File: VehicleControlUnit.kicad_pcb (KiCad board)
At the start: 4 copper layers, 95 x 100 mm, 99 parts, among them Con1 LED, Con2 LED, J1 Conn_01x02, J10 CAR_CAN_OUT, J11 CAR_CAN_Breakout, J12 USB_C_Receptacle_USB2.0_16P, J13 UART_Breakout, J14 Conn_01x04, J15 Conn_01x04, J16 IO_Breakout, J2 Precharge_Ready, J4 Precharge+_Conn, J5 Precharge-_Conn, J6 MOTOR_CAN_IN, J7 MOTOR_CAN_OUT, J8 MOTOR_CAN_Breakout, J9 CAR_CAN_IN, Q1 Q_PMOS_GDS, Q2 IRLML0030, Q3 IRLML0030, SW1 RESET, SW2 BOOT, U1 TLV1117LV33DCYR, U3 ESP32-C6-MINI-1/U, U4 TCMT1106, U5 TCMT1106

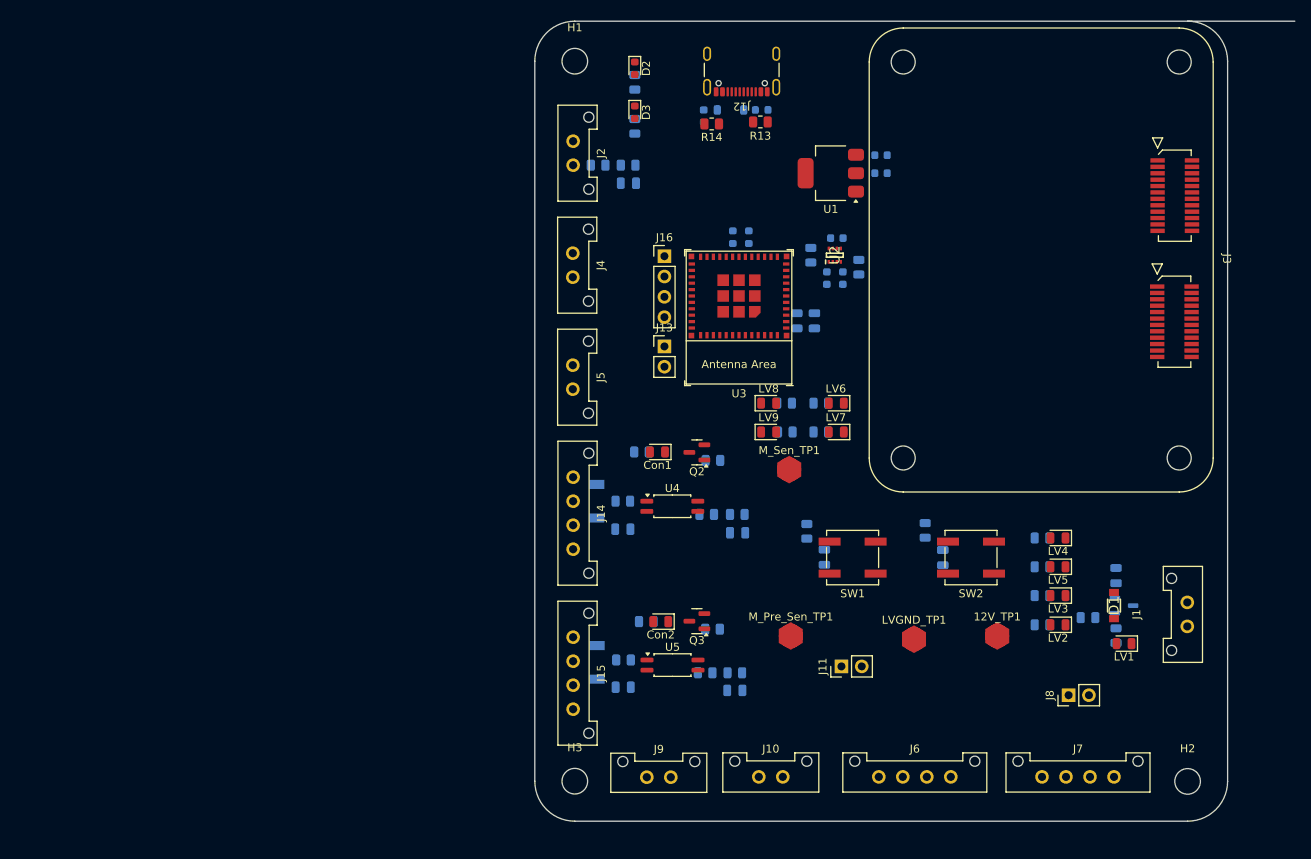
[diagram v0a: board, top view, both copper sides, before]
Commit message: first revision
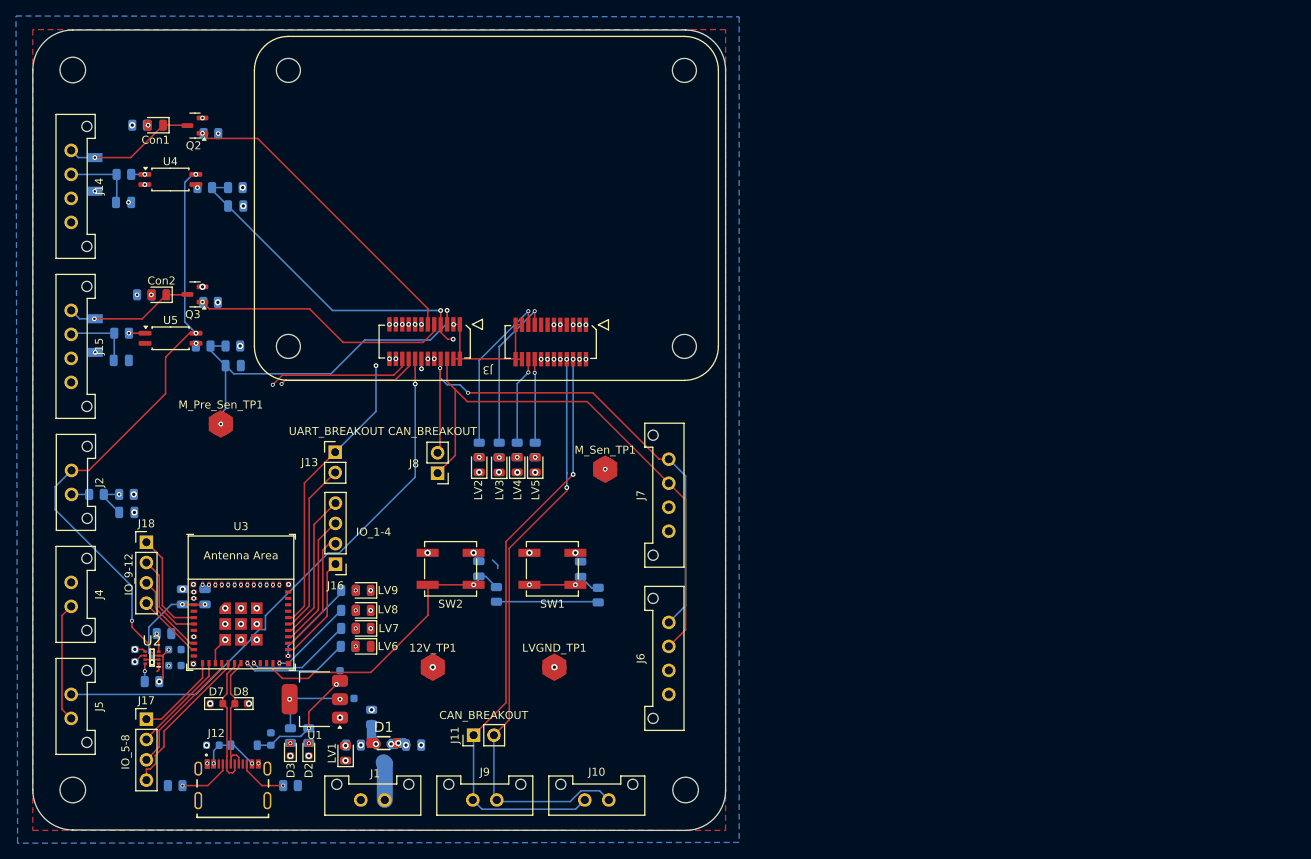
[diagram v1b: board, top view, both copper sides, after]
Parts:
- added J17: IO_5-8, Connector_PinHeader_2.54mm:PinHeader_1x04_P2.54mm_Vertical, F.Cu at (123.4, 128.0)
- added J18: IO_9-12, Connector_PinHeader_2.54mm:PinHeader_1x04_P2.54mm_Vertical, F.Cu at (123.4, 105.9)
- D7: renamed from D6; moved to F.Cu
- D8: renamed from D7; moved to F.Cu
- J12: footprint Connector_USB:USB_C_Receptacle_GCT_USB4105-xx-A_16P_TopMnt_Horizontal -> USBC:GCT_USB4215-03-A_REVA
- J16: value IO_Breakout -> IO_1-4
- R13, R14: moved to B.Cu
- moved J12 112.1 mm to (134.2, 138.2), turned to 0 degrees
- moved R13 110.6 mm to (127.0, 136.3), turned to 180 degrees
- moved J1 105.6 mm to (150.2, 138.1), turned to 0 degrees
- moved D6 104.9 mm to (131.8, 131.3), turned to 0 degrees
- moved C5 102.1 mm to (122.0, 120.1), turned to 90 degrees
- moved D4 100.0 mm to (135.7, 131.3), turned to 180 degrees
- moved U2 99.1 mm to (124.1, 120.3), turned to 180 degrees
- moved LV1 98.3 mm to (148.3, 132.2), turned to 90 degrees
- moved R11 98.2 mm to (125.6, 117.3), turned to 0 degrees
- moved R12 98.1 mm to (124.1, 123.3), turned to 180 degrees
- moved R14 98.0 mm to (141.5, 136.3), turned to 0 degrees
- moved R4 96.3 mm to (149.3, 131.2), turned to 180 degrees
- moved C3 95.5 mm to (127.0, 119.3), turned to 0 degrees
- moved C11 94.8 mm to (139.0, 130.5), turned to 90 degrees
- moved C9 94.8 mm to (127.0, 121.3), turned to 0 degrees
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- renumbered C10 to C11, C11 to C12, C12 to C13, C13 to C14, C14 to C15, C15 to C16, C16 to C17, D9 to D10, D5 to D6, D8 to D9
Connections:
- J3 pad 18: /VPrecharge+ -> /ISO_ADC_CLK
- J3 pad 20: /ISO_ADC_CLK -> /VPrecharge+
- U3 pad 10: unconnected-(U3-MTDI/GPIO5/ADC1_CH5-Pad10) -> /ESP/IO12
- U3 pad 12: unconnected-(U3-GPIO0/ADC1_CH0/XTAL_32K_P-Pad12) -> /ESP/IO5
- U3 pad 13: unconnected-(U3-GPIO1/ADC1_CH1/XTAL_32K_N-Pad13) -> /ESP/IO6
- U3 pad 15: unconnected-(U3-MTCK/GPIO6/ADC1_CH6-Pad15) -> /ESP/IO7
- U3 pad 16: unconnected-(U3-MTDO/GPIO7-Pad16) -> /ESP/IO8
- U3 pad 5: unconnected-(U3-GPIO2/ADC1_CH2-Pad5) -> /ESP/IO9
- U3 pad 6: unconnected-(U3-GPIO3/ADC1_CH3-Pad6) -> /ESP/IO10
- U3 pad 9: unconnected-(U3-MTMS/GPIO4/ADC1_CH4-Pad9) -> /ESP/IO11
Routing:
- net /3V3_LSOM: track 0.00 -> 133.8 mm, vias 0 -> 6
- net /C_CAN_H: track 0.00 -> 75.2 mm, vias 0 -> 2
- net /C_CAN_L: track 0.00 -> 74.1 mm, vias 0 -> 2
- net /ISO_ADC_CLK: track 0.00 -> 71.4 mm, vias 0 -> 1
- net /VPrecharge-: track 0.00 -> 70.2 mm, vias 0 -> 1
- net /M_CAN_H: track 0.00 -> 69.3 mm
- net /M_CAN_L: track 0.00 -> 68.0 mm, vias 0 -> 2
- net /M_Sense: track 0.00 -> 67.5 mm, vias 0 -> 3
- net /ESP/RESET: track 0.00 -> 56.0 mm, vias 0 -> 3
- net /VPrecharge+: track 0.00 -> 53.5 mm, vias 0 -> 1
- net /Precharge_Ready: track 0.00 -> 50.5 mm, vias 0 -> 2
- net /MPre_Sense: track 0.00 -> 46.8 mm, vias 0 -> 2
- net /ESP_RX: track 0.00 -> 45.7 mm, vias 0 -> 1
- net /ESP_TX: track 0.00 -> 42.9 mm, vias 0 -> 2
- net /M_Enable: track 0.00 -> 39.2 mm, vias 0 -> 1
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- added copper zone on B.Cu, net GND
- added copper zone on F.Cu, net GND
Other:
- board size 95 x 100 mm -> 86.6 x 100.1 mm
- board text added: "CAN_BREAKOUT"
- board text added: "UART_BREAKOUT"
